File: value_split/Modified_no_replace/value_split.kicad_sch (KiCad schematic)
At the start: 6 parts

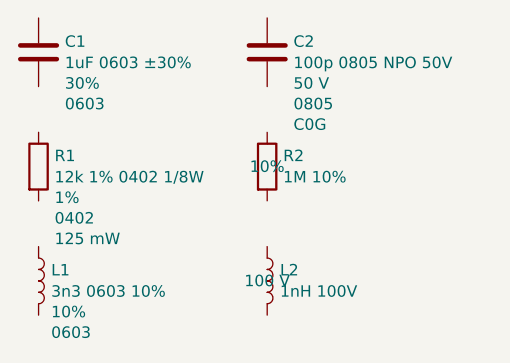
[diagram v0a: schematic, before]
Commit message: KiBot generated updated
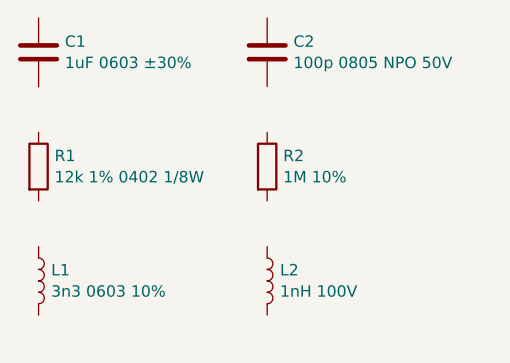
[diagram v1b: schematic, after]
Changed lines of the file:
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@@
     )
     (property "tolerance" "30%" (id 4) (at 79.121 58.0644 0)
-      (effects (font (size 1.27 1.27)) (justify left))
+      (effects (font (size 1.27 1.27)) (justify left) hide)
     )
     (property "package" "0603" (id 5) (at 79.121 60.3504 0)
-      (effects (font (size 1.27 1.27)) (justify left))
+      (effects (font (size 1.27 1.27)) (justify left) hide)
     )
     (pin "1")
@@
     )
     (property "voltage" "50 V" (id 4) (at 104.521 58.0644 0)
-      (effects (font (size 1.27 1.27)) (justify left))
+      (effects (font (size 1.27 1.27)) (justify left) hide)
     )
     (property "package" "0805" (id 5) (at 104.521 60.3504 0)
-      (effects (font (size 1.27 1.27)) (justify left))
+      (effects (font (size 1.27 1.27)) (justify left) hide)
     )
     (property "temp_coef" "C0G" (id 6) (at 104.521 62.6364 0)
-      (effects (font (size 1.27 1.27)) (justify left))
+      (effects (font (size 1.27 1.27)) (justify left) hide)
     )
     (pin "1")
@@
     )
     (property "tolerance" "1%" (id 4) (at 77.978 70.7644 0)
-      (effects (font (size 1.27 1.27)) (justify left))
+      (effects (font (size 1.27 1.27)) (justify left) hide)
     )
     (property "package" "0402" (id 5) (at 77.978 73.0504 0)
-      (effects (font (size 1.27 1.27)) (justify left))
+      (effects (font (size 1.27 1.27)) (justify left) hide)
     )
     (property "power" "125 mW" (id 6) (at 77.978 75.3364 0)
-      (effects (font (size 1.27 1.27)) (justify left))
+      (effects (font (size 1.27 1.27)) (justify left) hide)
     )
     (pin "1")
@@
     )
     (property "tolerance" "10%" (id 4) (at 101.6 67.31 0)
-      (effects (font (size 1.27 1.27)))
+      (effects (font (size 1.27 1.27)) hide)
     )
     (pin "1")
@@
     )
     (property "tolerance" "10%" (id 4) (at 77.597 83.4644 0)
-      (effects (font (size 1.27 1.27)) (justify left))
+      (effects (font (size 1.27 1.27)) (justify left) hide)
     )
     (property "package" "0603" (id 5) (at 77.597 85.7504 0)
-      (effects (font (size 1.27 1.27)) (justify left))
+      (effects (font (size 1.27 1.27)) (justify left) hide)
     )
     (pin "1")
@@
     )
     (property "Voltage" "100 V" (id 4) (at 101.6 80.01 0)
-      (effects (font (size 1.27 1.27)))
+      (effects (font (size 1.27 1.27)) hide)
     )
     (pin "1")
